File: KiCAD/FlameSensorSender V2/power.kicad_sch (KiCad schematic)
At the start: 17 parts, among them IC1 LM66200DRLR, J7 Conn_01x06_Socket, J8 Conn_01x04_Pin, J9 6 Pin USB-C Type USB Connecto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, P1 XL638020, P2 XL638020, Q5 AO3400A, Q6 AO3401A, U3 TVS0500DRV

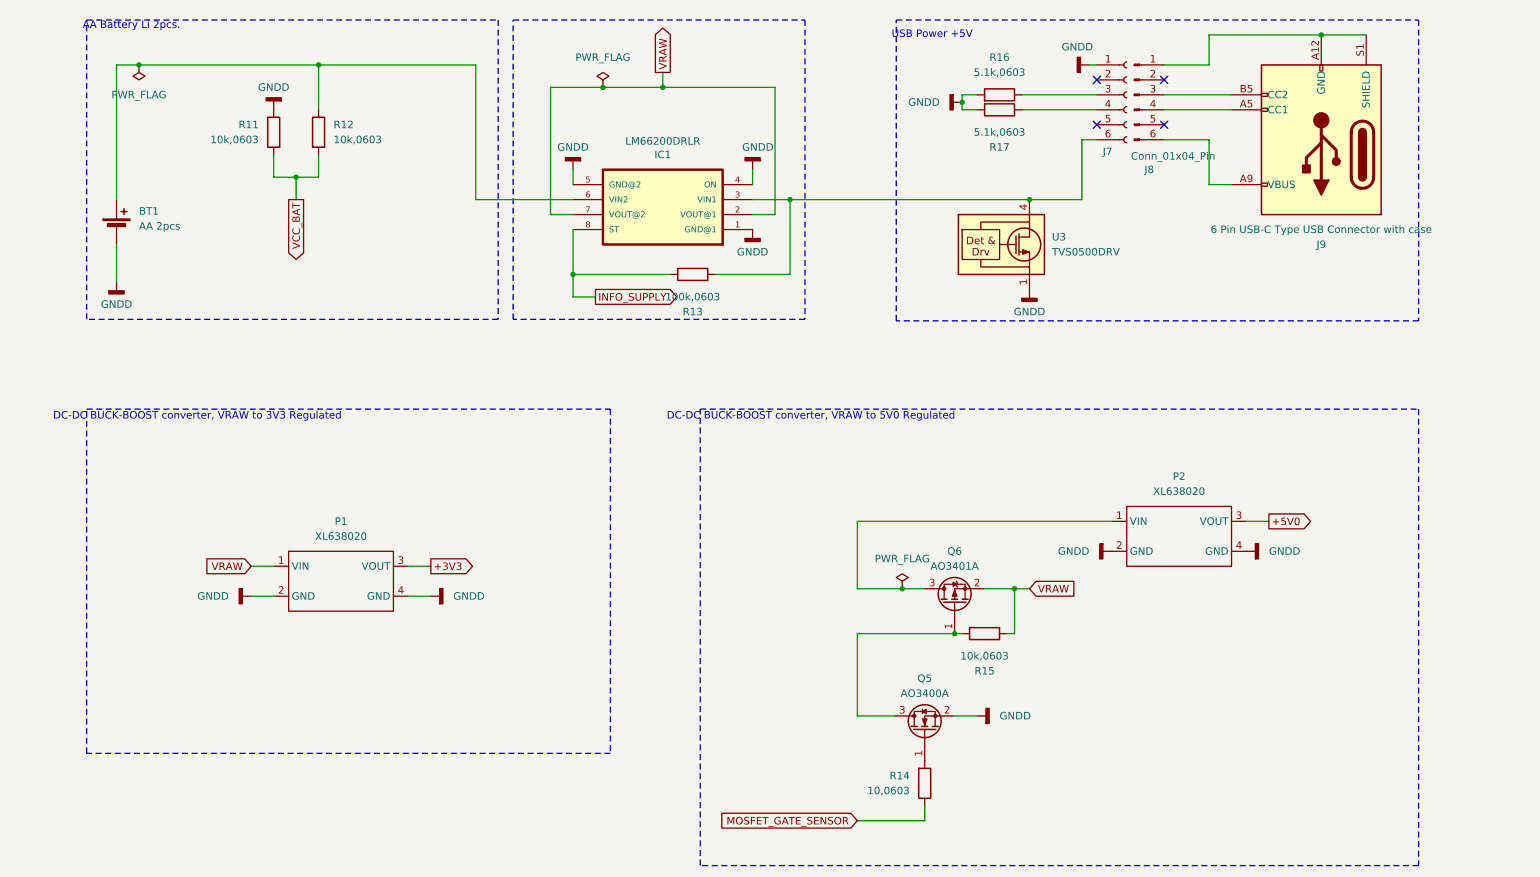
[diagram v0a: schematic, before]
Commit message: dev
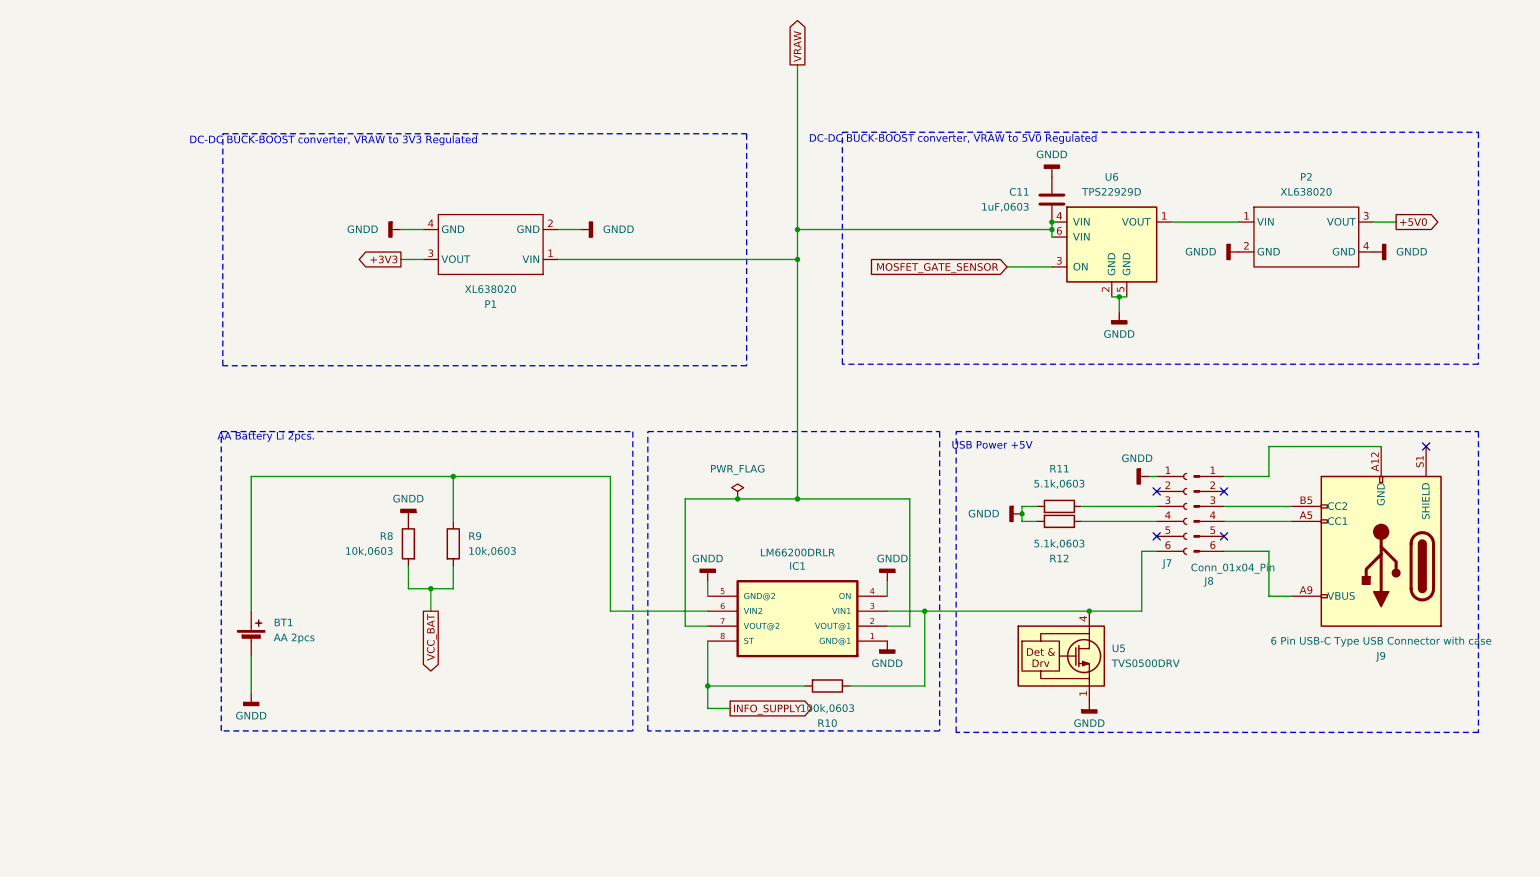
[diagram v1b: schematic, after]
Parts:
- removed Q5: AO3400A, Package_TO_SOT_SMD:SOT-23, symbol Transistor_FET:AO3400A
- removed Q6: AO3401A, Package_TO_SOT_SMD:SOT-23-3, symbol Transistor_FET:AO3401A
- removed R14: 10,0603, Resistor_SMD:R_0603_1608Metric_Pad0.98x0.95mm_HandSolder, symbol Device:R
- removed R15: 10k,0603, Resistor_SMD:R_0603_1608Metric_Pad0.98x0.95mm_HandSolder, symbol Device:R
- added C11: 1uF,0603, Capacitor_SMD:C_0603_1608Metric_Pad1.08x0.95mm_HandSolder, symbol Device:C
- added U6: TPS22929D, Package_TO_SOT_SMD:SOT-23-6, symbol Power_Management:TPS22929D
- renumbered R13 to R10, R16 to R11, R17 to R12, R11 to R8, R12 to R9, U3 to U5
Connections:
- net GNDD: now also C11.2, U6.2 (GND), U6.5 (GND)
- net MOSFET_GATE_SENSOR: now also U6.3 (ON)
- net VRAW: now also C11.1, U6.4 (VIN), U6.6 (VIN)
- net at P2.1 (VIN): now also U6.1 (VOUT)
- net at J8.1 (Pin_1), J9.A12 (GND), J9.B12 (GND): no longer J9.S1 (SHIELD)
- no-connect marks 4 -> 5
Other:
- moved on the sheet: BT1, IC1, J7, J8, J9, P1, P2, R10, R11, R12, R8, R9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
